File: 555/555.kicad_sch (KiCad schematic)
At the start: 6 parts, among them U1 NE555P

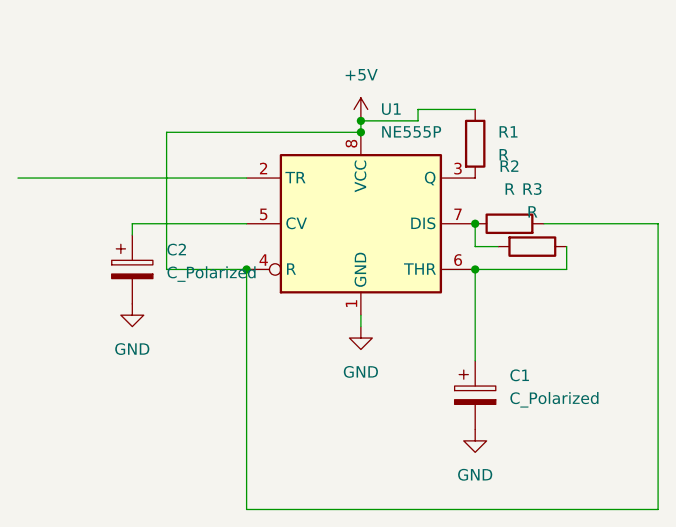
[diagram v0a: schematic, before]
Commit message: pcb
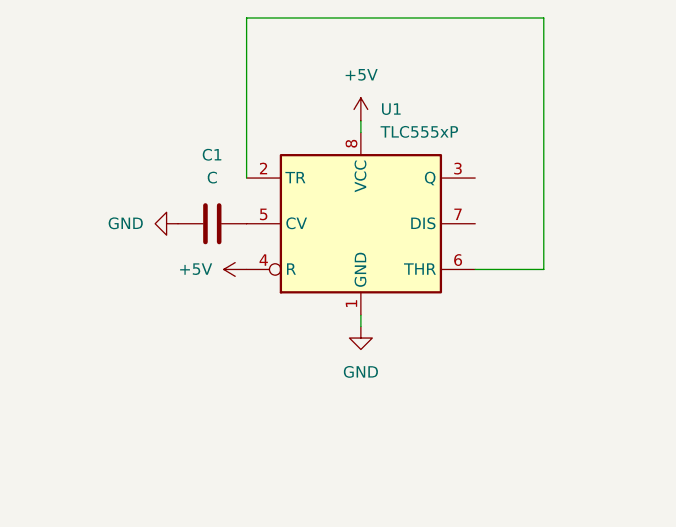
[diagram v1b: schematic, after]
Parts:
- removed C1, C2: C_Polarized, symbol Device:C_Polarized
- removed R1, R2, R3: R, symbol Device:R
- removed U1: NE555P, Package_DIP:DIP-8_W7.62mm, symbol Timer:NE555P
- added C1: C, symbol Device:C
- added U1: TLC555xP, Package_SO:SOIC-8_3.9x4.9mm_P1.27mm, symbol Timer:TLC555xP
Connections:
- net +5V: now also U1.4 (R), U1.8 (VCC)
- net GND: now also C1.1, U1.1 (GND)
- new net: C1.2, U1.5 (CV)
- new net: U1.2 (TR), U1.6 (THR)
